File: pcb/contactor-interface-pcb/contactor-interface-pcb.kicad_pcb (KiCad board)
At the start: 2 copper layers, 40.6 x 29.1 mm, 13 parts, among them J1 Conn_01x04_Socket, K1 G3MB-202PDC5

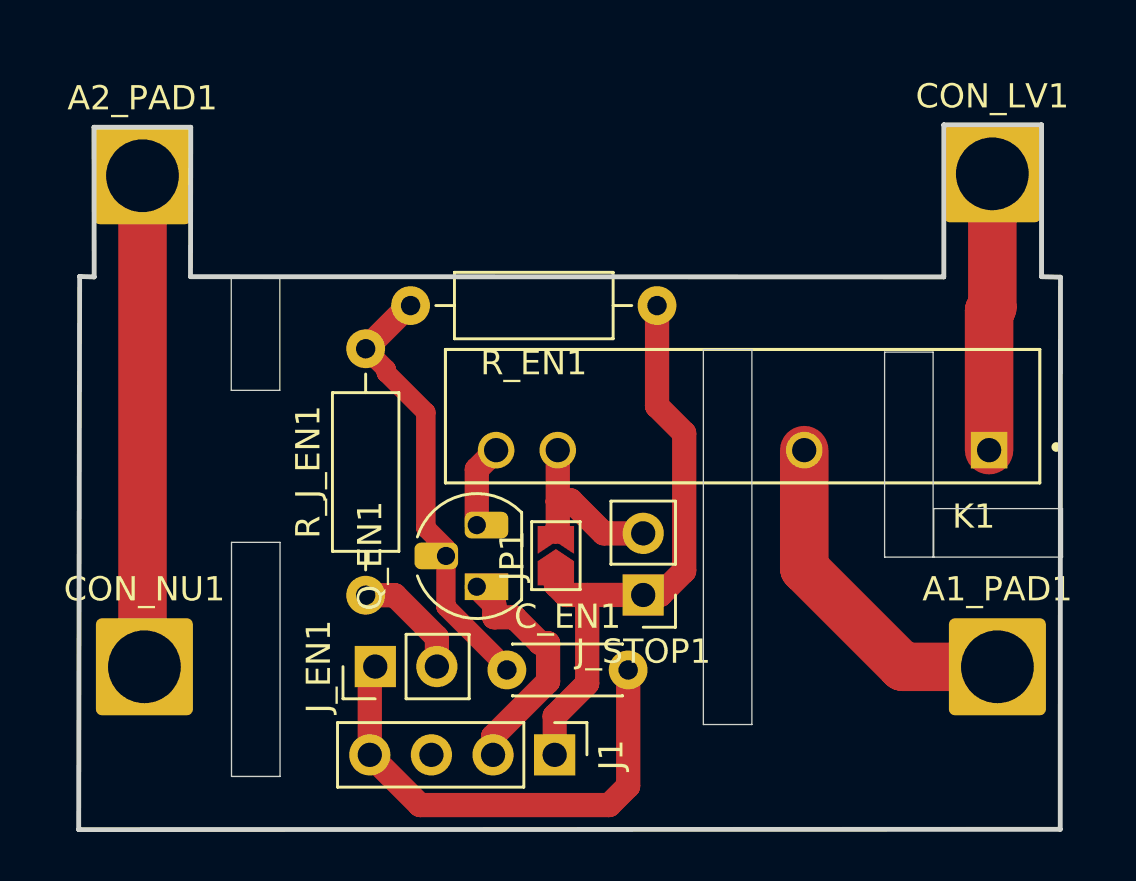
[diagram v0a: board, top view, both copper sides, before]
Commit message: Progress with SMT controller and contactor variant
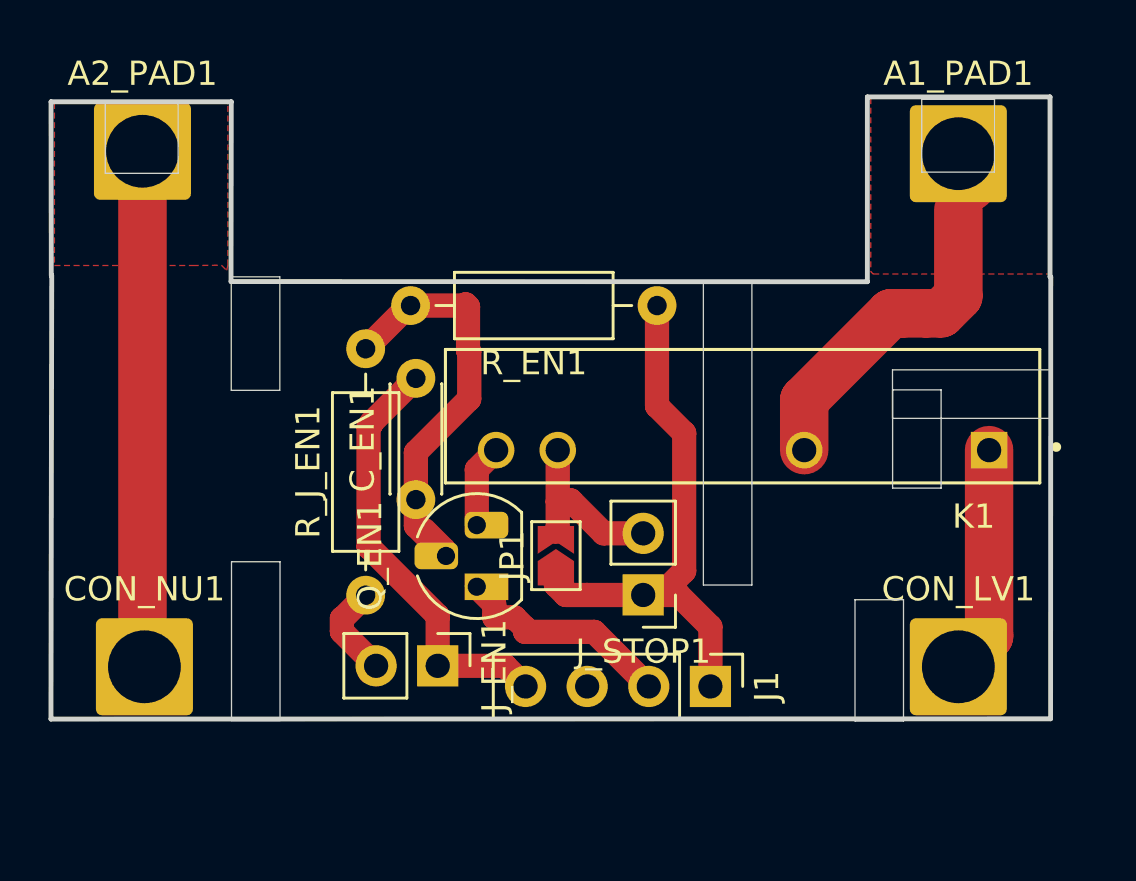
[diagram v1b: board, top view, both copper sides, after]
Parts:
- moved A1_PAD1 21.3 mm to (36.2, 1.50)
- moved CON_LV1 20.4 mm to (36.2, 22.8)
- moved C_EN1 7.96 mm to (13.8, 15.9), turned to 90 degrees
- moved J1 7.01 mm to (26.0, 23.6)
- moved J_EN1 2.58 mm to (14.7, 22.7), turned to -90 degrees
- moved A2_PAD1 1.01 mm to (2.57, 1.50)
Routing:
- net GND: track 20.4 -> 17.8 mm
- net Net-(CON_LV1-Pin_1): track 11.4 -> 9.46 mm
- net +5V: track 24.9 -> 23.5 mm
- net Net-(J_EN1-Pin_2): track 4.86 -> 4.27 mm
- net Net-(J1-Pin_2): track 9.76 -> 9.20 mm
- added copper zone on F.Cu, net Net-(A1_PAD1-Pin_1)
- added copper zone on F.Cu, net Net-(A2_PAD1-Pin_1)
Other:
- board size 40.6 x 29.1 mm -> 41.2 x 25.7 mm
